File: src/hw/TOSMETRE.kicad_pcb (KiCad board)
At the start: 2 copper layers, 4.5 x 3.5 mm, 61 parts, among them J1 Barrel_Jack_Switch, J2 Conn_01x02_Male, J3 Conn_01x08_Male, J4 Conn_Coaxial, J5 Conn_01x05_Male, J6 Conn_01x02_Male, J7 Conn_Coaxial, SW1 SW_DIP_x01, U1 TPS70950DBVT, U2 18F1320, U3 LT1818, U4 LTC2305, U5 LT1818

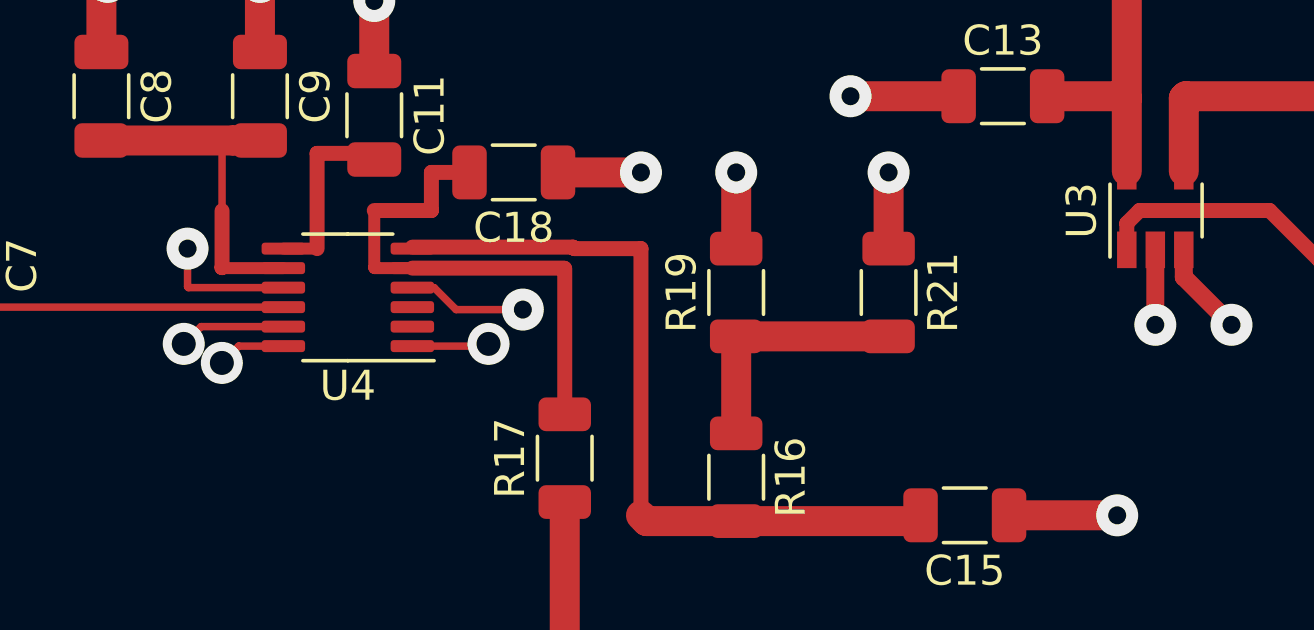
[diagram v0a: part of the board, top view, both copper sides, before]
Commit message: #305
Livraison suite a coup de telephone
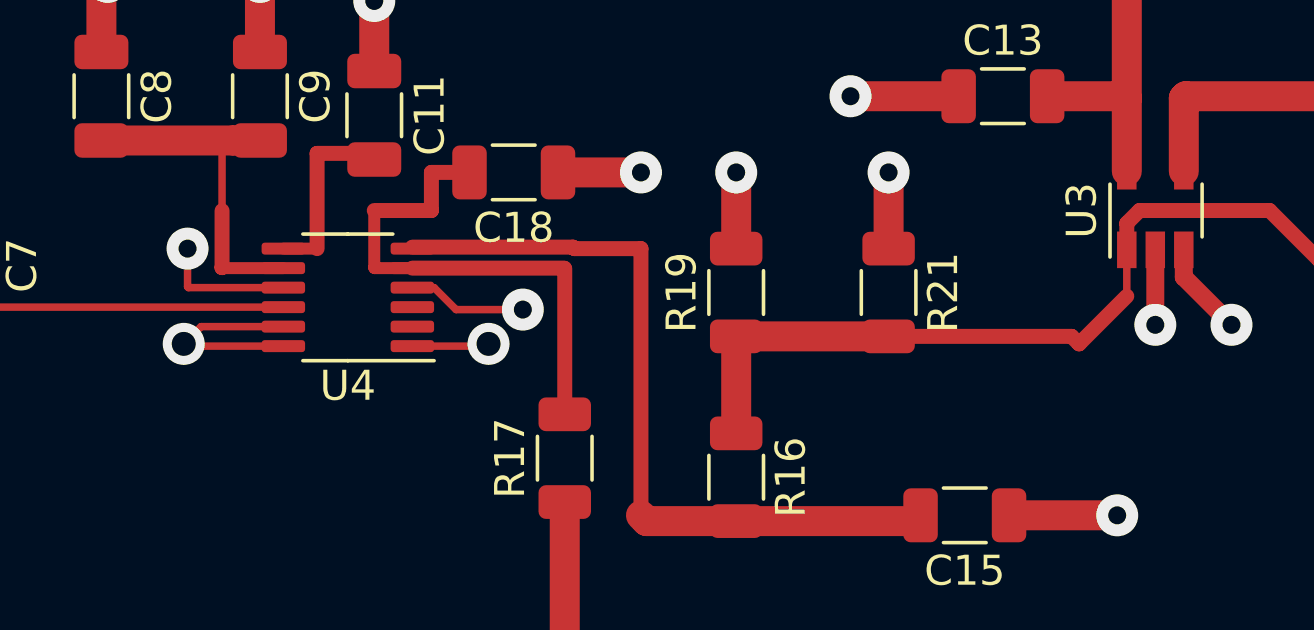
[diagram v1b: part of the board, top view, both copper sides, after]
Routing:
- net Net-(R16-Pad1): track 20.5 -> 30.7 mm
- net GNDREF: track 150.4 -> 151.5 mm, vias 47 -> 46
